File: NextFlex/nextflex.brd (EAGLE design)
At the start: 160 x 100 mm, 46 parts, among them J1 FFC-32, J8 FFC-32, U1 DG406DYZ-T, U2 DG406DYZ-T, U3 AD5933YRSZ, U4 AFE4490_AFE4490, U5 AZ1117EH-3.3TRG1, U6 LM340SX-5.0/NOPB

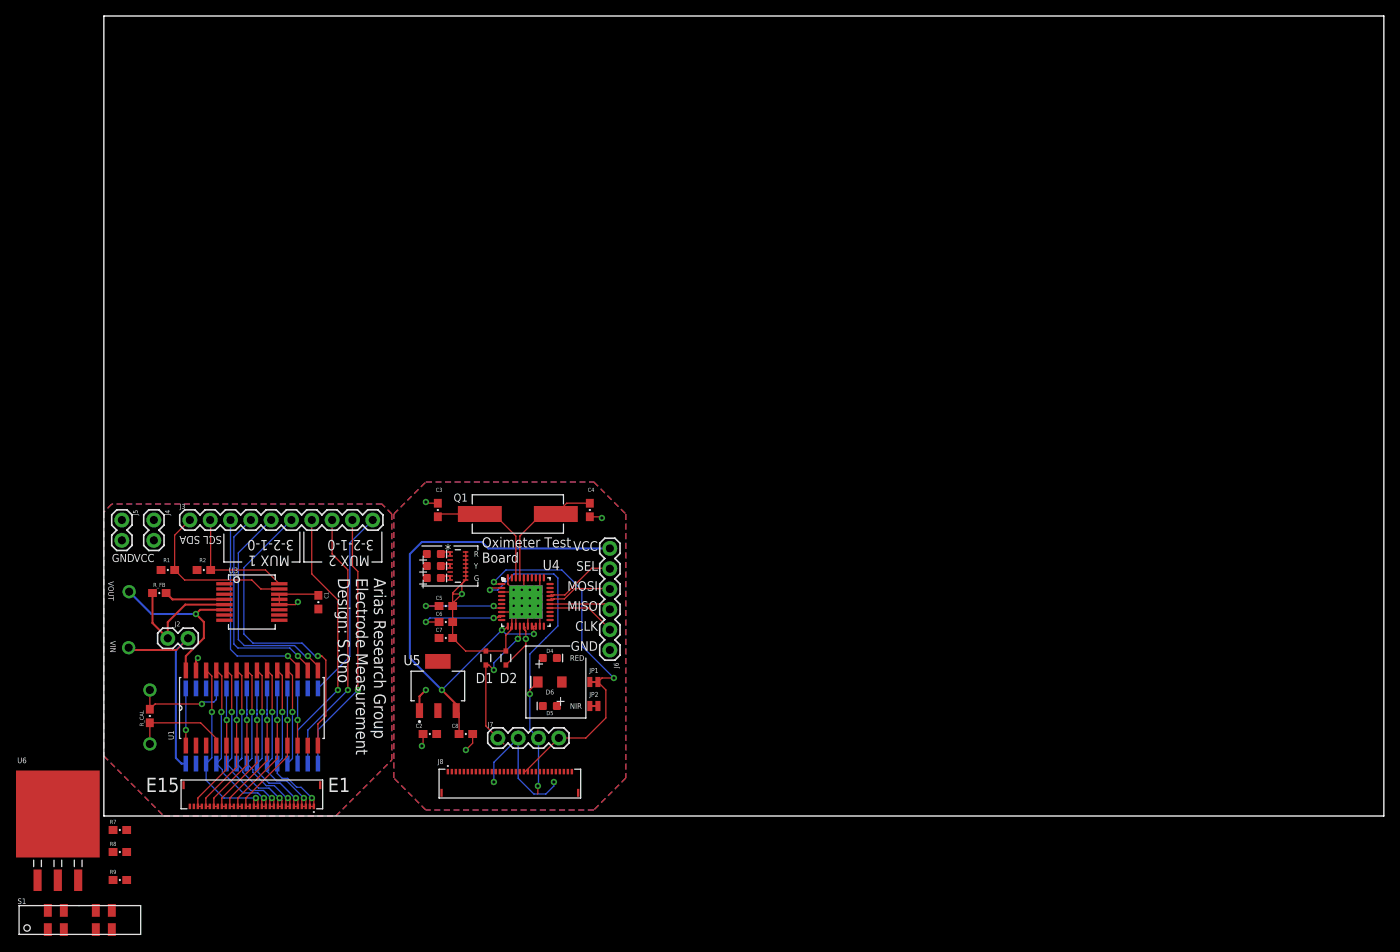
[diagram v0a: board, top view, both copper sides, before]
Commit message: finish rev a of nextflex
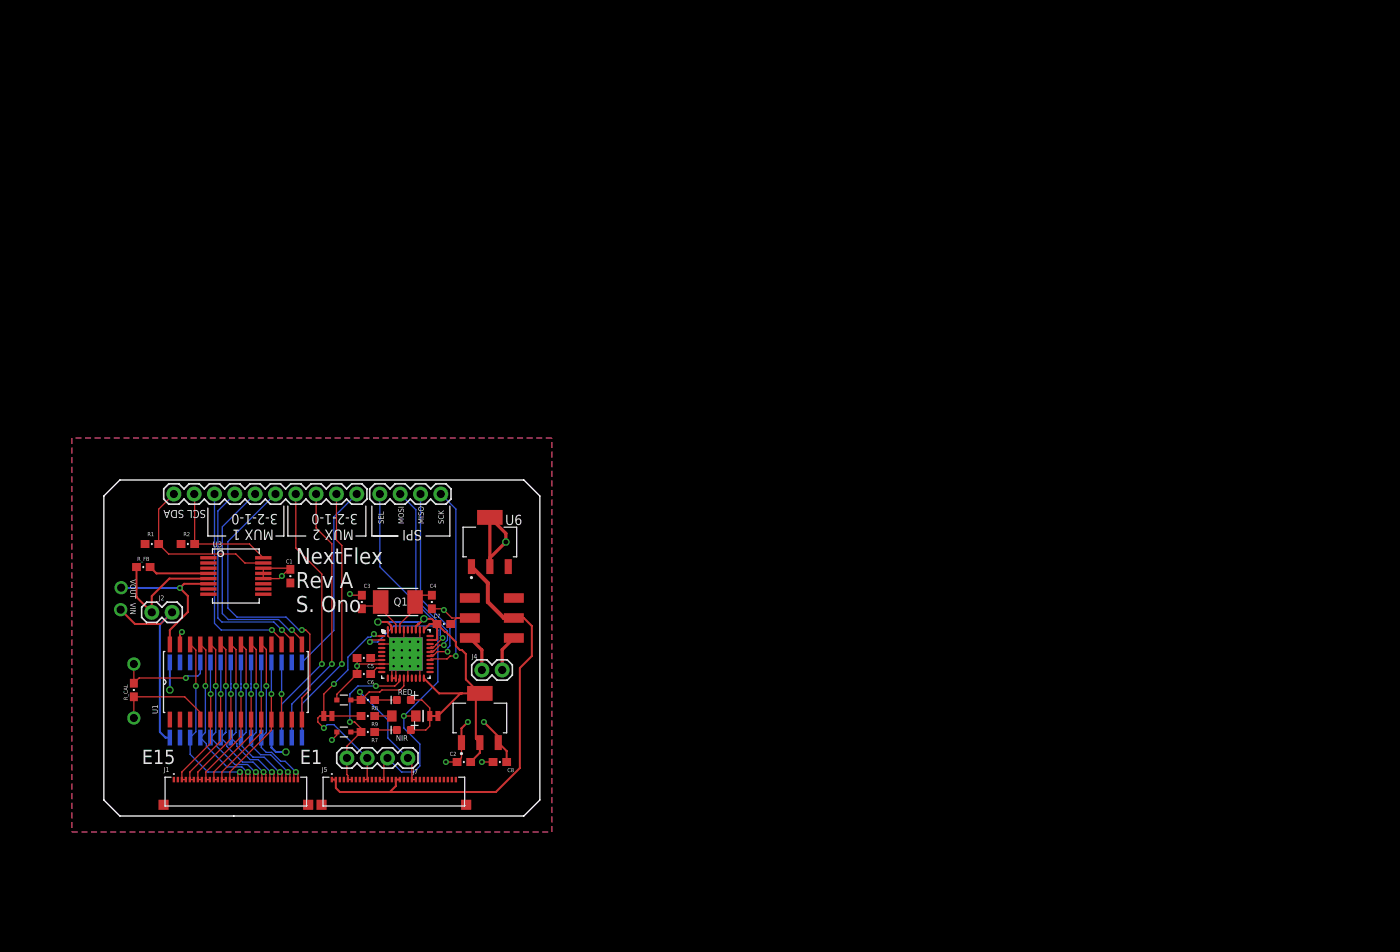
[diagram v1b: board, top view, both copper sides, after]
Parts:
- removed D7: RED, scono:LED-0603
- removed D8: YELLOW, scono:LED-0603
- removed D9: GREEN, scono:LED-0603
- removed J8: FFC-32, scono:MOLEX_503480-3200
- removed R3: 330R, scono:EXB2HV
- removed S1: (no value), scono:DP3T
- added S2: DPDT-SWITCH, scono:SW_JS202011SCQN
- J4: value (none) -> BAT
- J5: value (none) -> FFC-32; device scono:1X02 -> scono:MOLEX_503480-3200
- J6: device scono:1X06 -> scono:1X04
- Q1: device scono:XTAL_ECS-80-18-5PX-TR -> scono:XTAL500X320X130N
- U6: value LM340SX-5.0/NOPB -> LM340MPX-5.0230; device scono:TS3B -> scono:SOT230P700X180-4N
- moved U6 63.8 mm to (48.2, 34.2), turned to 90 degrees
- moved J5 48.3 mm to (36.2, 2.75), turned to 0 degrees
- moved J4 45.1 mm to (47.2, 18.2), turned to 0 degrees
- moved R9 37.2 mm to (33.0, 12.5), turned to 180 degrees
- moved R8 36.4 mm to (33.0, 14.5), turned to 180 degrees
- moved J6 34.7 mm to (34.5, 40.2), turned to 0 degrees
- moved JP1 33.5 mm to (28.0, 12.5), turned to 180 degrees
- moved R7 33.3 mm to (33.0, 10.5), turned to 180 degrees
- moved C4 22.9 mm to (41.0, 26.8)
- moved D2 20.9 mm to (30.0, 14.5), turned to 180 degrees
- moved JP2 20.0 mm to (41.2, 12.5)
- moved D1 20.0 mm to (30.0, 10.5), turned to 180 degrees
- moved D4 19.0 mm to (37.5, 14.5), turned to 180 degrees
- moved D6 18.7 mm to (37.5, 12.5), turned to 0 degrees
- moved Q1 18.6 mm to (36.8, 26.8)
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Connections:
- removed net 9V: J8.11, J8.12, J8.27, J8.28
- removed net GRN: D9.A
- removed net IN: U6.1
- removed net N$5: D7.C, R3.1, R3.2
- removed net N$6: D8.C, R3.4, R3.5
- removed net N$7: D9.C, R3.7, R3.8
- removed net OUT: U6.3
- removed net YEL: D8.A
- new net BAT+: J4.2, S2.1
- new net BAT-: J4.1, S2.4
- net 3.3V: no longer D7.A
- net 5V: now also C1.2, R1.2, R2.2, U1.1, U1.18, U2.1, U2.18, U3.10, U3.11, U3.9, U6.3; no longer J6.6
- net E1: now also J1.31, J1.32; no longer J1.1, J1.2
- net E10: now also J1.13, J1.14; no longer J1.19, J1.20
- net E11: now also J1.11, J1.12; no longer J1.21, J1.22
- net E12: now also J1.10, J1.9; no longer J1.23, J1.24
- net E13: now also J1.7, J1.8; no longer J1.25, J1.26
- net E14: now also J1.5, J1.6; no longer J1.27, J1.28
- net E15: now also J1.3, J1.4; no longer J1.29, J1.30
- net E2: now also J1.29, J1.30; no longer J1.3, J1.4
- net E3: now also J1.27, J1.28; no longer J1.5, J1.6
- net E4: now also J1.25, J1.26; no longer J1.7, J1.8
- net E5: now also J1.23, J1.24; no longer J1.10, J1.9
- net E6: now also J1.21, J1.22; no longer J1.11, J1.12
- net E7: now also J1.19, J1.20; no longer J1.13, J1.14
- net E8: now also J1.17, J1.18; no longer J1.15, J1.16
- net E9: now also J1.15, J1.16; no longer J1.17, J1.18
- net GND: now also S2.5; no longer J5.1, J5.2, J6.1, R3.10, R3.11, R3.12, R3.13, R3.14, R3.15, R3.16, R3.9
- net INN: now also J5.10, J5.9, J7.3; no longer J7.4, J8.19, J8.20
- net INP: now also J5.13, J5.14, J7.2; no longer J7.3, J8.23, J8.24
- net SPI_MOSI: now also J6.2; no longer J6.4
- net SPI_SCLK: now also J6.4; no longer J6.2
- net SPI_SEL: now also J6.1; no longer J6.5
- net TXN: now also J5.5, J5.6, J7.4; no longer J7.1, J8.15, J8.16
- net TXP: now also J5.21, J5.22, J7.1; no longer J7.2, J8.31, J8.32
- net VCC: now also J5.1, J5.17, J5.18, J5.2, S2.2, U6.1; no longer C1.2, J4.1, J4.2, R1.2, R2.2, U1.1, U1.18, U2.1, U2.18, U3.10, U3.11, U3.9
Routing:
- net 5V: track 68.3 -> 12.9 mm
- net 3.3V: track 0.00 -> 49.3 mm, vias 0 -> 2
- net VCC: track 19.3 -> 59.0 mm, vias 2 -> 0
- net INN: track 46.6 -> 27.1 mm, vias 2 -> 3
- net SPI_MISO: track 7.75 -> 23.8 mm, vias 0 -> 1
- net SPI_SCLK: track 8.62 -> 24.5 mm, vias 0 -> 1
- net SPI_MOSI: track 8.10 -> 23.6 mm, vias 0 -> 1
- net SPI_SEL: track 8.94 -> 23.4 mm, vias 0 -> 1
- net TX_REF: track 11.4 -> 1.69 mm, vias 2 -> 0
- net BG: track 11.2 -> 1.48 mm, vias 2 -> 0
- net XIN: track 16.3 -> 8.17 mm
- net XOUT: track 15.7 -> 7.92 mm
- net N$16: track 0.00 -> 7.61 mm
- net GND: track 95.6 -> 101.7 mm, vias 9 -> 11
- net BAT-: track 0.00 -> 4.62 mm
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- added copper zone on layer 1, net 5V
- removed copper zone on layer 1, net 3.3V
- removed copper zone on layer 1, net VCC
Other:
- board size 160 x 100 mm -> 54.5 x 42 mm
- board text added: "Arias Research Group"
- board text added: "NextFlex Rev A S. Ono"
- board text added: "SCK"
- board text added: "SPI"
- board text removed: "Arias Research Group Electrode Measurement Design: S.Ono"
- board text removed: "CLK"
- board text removed: "G"
- board text removed: "GND"
- board text removed: "Oximeter Test Board"
- board text removed: "R"
- board text removed: "Seiya Ono Fa'19 NextFlex Prototype"
- board text removed: "VCC"
- board text removed: "Y"
